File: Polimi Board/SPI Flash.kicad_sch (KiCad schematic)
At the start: 1 part, among them IC1 M95512-RMN6P

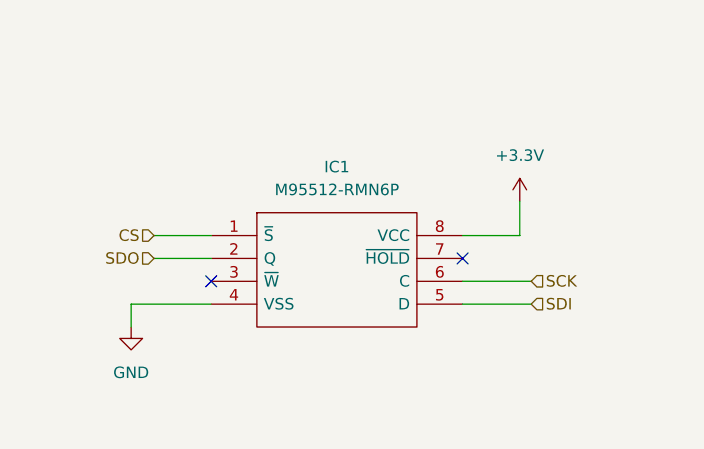
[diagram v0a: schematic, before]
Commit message: Fatte modifiche
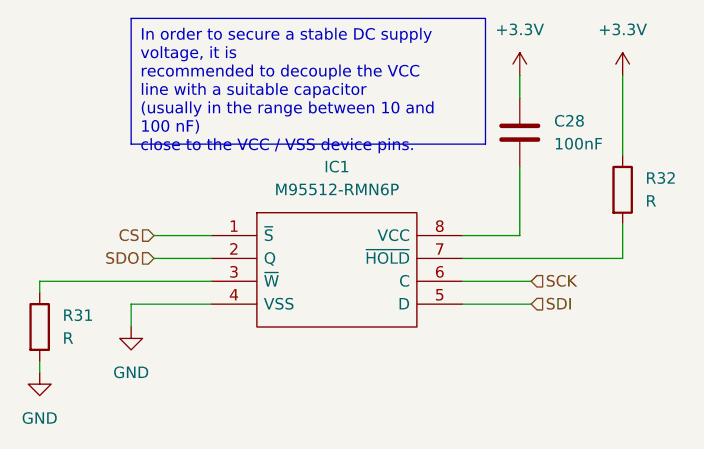
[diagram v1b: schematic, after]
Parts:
- added C28: 100nF, symbol Device:C
- added R31, R32: R, symbol Device:R
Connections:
- net +3.3V: now also C28.1, R32.1; no longer IC1.8 (VCC)
- net GND: now also R31.2
- net at IC1.3 (~{W}): now also R31.1
- net at IC1.7 (~{HOLD}): now also R32.2
- new net: C28.2, IC1.8 (VCC)
- no-connect marks 2 -> 0
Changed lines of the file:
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@@
   (title_block
     (title "Polimi Board ")
-    (date "2024-04-24")
-    (rev "1.0")
+    (date "2024-04-29")
+    (rev "2.0")
     (company "Politecnico di Milano")
     (comment 1 "Embedded Systems Project")
     (comment 2 "ing. Zaccaria Eliseo Carrettoni")
   )
-  (no_connect (at 125.73 92.71))
-  (no_connect (at 153.67 90.17))
+  (wire (pts (xy 153.67 90.17) (xy 171.45 90.17))
+    (stroke (width 0) (type default))
+  )
   (wire (pts (xy 153.67 87.63) (xy 160.02 87.63))
     (stroke (width 0) (type default))
@@
     (stroke (width 0) (type default))
   )
+  (wire (pts (xy 171.45 90.17) (xy 171.45 86.36))
+    (stroke (width 0) (type default))
+  )
+  (wire (pts (xy 106.68 101.6) (xy 106.68 102.87))
+    (stroke (width 0) (type default))
+  )
+  (wire (pts (xy 106.68 93.98) (xy 106.68 92.71))
+    (stroke (width 0) (type default))
+  )
+  (wire (pts (xy 171.45 69.85) (xy 171.45 78.74))
+    (stroke (width 0) (type default))
+  )
   (wire (pts (xy 119.38 87.63) (xy 125.73 87.63))
     (stroke (width 0) (type default))
@@
     (stroke (width 0) (type default))
   )
-  (wire (pts (xy 160.02 83.82) (xy 160.02 87.63))
+  (wire (pts (xy 160.02 72.39) (xy 160.02 69.85))
+    (stroke (width 0) (type default))
+  )
+  (wire (pts (xy 106.68 92.71) (xy 125.73 92.71))
+    (stroke (width 0) (type default))
+  )
+  (wire (pts (xy 160.02 80.01) (xy 160.02 87.63))
     (stroke (width 0) (type default))
   )
   (wire (pts (xy 116.84 97.79) (xy 116.84 95.25))
     (stroke (width 0) (type default))
+  )
+  (text_box "In order to secure a stable DC supply voltage, it is\nrecommended to decouple the VCC line with a suitable capacitor (usually in the range between 10 and 100 nF)\nclose to the VCC / VSS device pins."
+    (at 116.84 63.5 0) (size 39.37 13.97)
+    (stroke (width 0) (type default))
+    (fill (type none))
+    (effects (font (size 1.27 1.27)) (justify left top))
   )
   (hierarchical_label "SDI" (shape input) (at 161.29 95.25 0) (fields_autoplaced)
@@
         (path "/319fe76e-1f98-44b3-99b0-af1a9ad7322c/6ede4352-cbae-4369-81ad-e8e15f2edc14"
           (reference "#PWR018") (unit 1)
-        )
-      )
-    )
-  )
-  (symbol (lib_id "power:+3.3V") (at 160.02 83.82 0) (unit 1)
-    (in_bom yes) (on_board yes) (dnp no) (fields_autoplaced)
-    (property "Reference" "#PWR053" (at 160.02 87.63 0)
-      (effects (font (size 1.27 1.27)) hide)
-    )
-    (property "Value" "+3.3V" (at 160.02 78.74 0)
-      (effects (font (size 1.27 1.27)))
-    )
-    (property "Footprint" "" (at 160.02 83.82 0)
-      (effects (font (size 1.27 1.27)) hide)
-    )
-    (property "Datasheet" "" (at 160.02 83.82 0)
-      (effects (font (size 1.27 1.27)) hide)
-    )
-    (pin "1")
-    (instances
-      (project "Polimi Board"
-        (path "/319fe76e-1f98-44b3-99b0-af1a9ad7322c/6ede4352-cbae-4369-81ad-e8e15f2edc14"
-          (reference "#PWR053") (unit 1)
         )
       )
@@
         )
       )
+    )
+  )
+  (symbol (lib_id "Device:C") (at 160.02 76.2 0) (unit 1)
+    (in_bom yes) (on_board yes) (dnp no) (fields_autoplaced)
+    (property "Reference" "C28" (at 163.83 74.93 0)
+      (effects (font (size 1.27 1.27)) (justify left))
+    )
+    (property "Value" "100nF" (at 163.83 77.47 0)
+      (effects (font (size 1.27 1.27)) (justify left))
+    )
+    (property "Footprint" "" (at 160.9852 80.01 0)
+      (effects (font (size 1.27 1.27)) hide)
+    )
+    (property "Datasheet" "~" (at 160.02 76.2 0)
+      (effects (font (size 1.27 1.27)) hide)
+    )
+    (pin "2")
+    (pin "1")
+    (instances
+      (project "Polimi Board"
+        (path "/319fe76e-1f98-44b3-99b0-af1a9ad7322c/6ede4352-cbae-4369-81ad-e8e15f2edc14"
+          (reference "C28") (unit 1)
+        )
+      )
+    )
+  )
+  (symbol (lib_id "Device:R") (at 106.68 97.79 0) (unit 1)
+    (in_bom yes) (on_board yes) (dnp no) (fields_autoplaced)
+    (property "Reference" "R31" (at 109.22 96.52 0)
+      (effects (font (size 1.27 1.27)) (justify left))
+    )
+    (property "Value" "R" (at 109.22 99.06 0)
+      (effects (font (size 1.27 1.27)) (justify left))
+    )
+    (property "Footprint" "" (at 104.902 97.79 90)
+      (effects (font (size 1.27 1.27)) hide)
+    )
+    (property "Datasheet" "~" (at 106.68 97.79 0)
+      (effects (font (size 1.27 1.27)) hide)
+    )
+    (pin "1")
+    (pin "2")
+    (instances
+      (project "Polimi Board"
+        (path "/319fe76e-1f98-44b3-99b0-af1a9ad7322c/6ede4352-cbae-4369-81ad-e8e15f2edc14"
+          (reference "R31") (unit 1)
+        )
+      )
+    )
+  )
+  (symbol (lib_id "power:+3.3V") (at 160.02 69.85 0) (unit 1)
+    (in_bom yes) (on_board yes) (dnp no) (fields_autoplaced)
+    (property "Reference" "#PWR025" (at 160.02 73.66 0)
+      (effects (font (size 1.27 1.27)) hide)
+    )
+    (property "Value" "+3.3V" (at 160.02 64.77 0)
+      (effects (font (size 1.27 1.27)))
+    )
+    (property "Footprint" "" (at 160.02 69.85 0)
+      (effects (font (size 1.27 1.27)) hide)
+    )
+    (property "Datasheet" "" (at 160.02 69.85 0)
+      (effects (font (size 1.27 1.27)) hide)
+    )
+    (pin "1")
+    (instances
+      (project "Polimi Board"
+        (path "/319fe76e-1f98-44b3-99b0-af1a9ad7322c/6ede4352-cbae-4369-81ad-e8e15f2edc14"
+          (reference "#PWR025") (unit 1)
+        )
+      )
+    )
+  )
+  (symbol (lib_id "power:GND") (at 106.68 102.87 0) (unit 1)
+    (in_bom yes) (on_board yes) (dnp no) (fields_autoplaced)
+    (property "Reference" "#PWR069" (at 106.68 109.22 0)
+      (effects (font (size 1.27 1.27)) hide)
+    )
+    (property "Value" "GND" (at 106.68 107.95 0)
+      (effects (font (size 1.27 1.27)))
+    )
+    (property "Footprint" "" (at 106.68 102.87 0)
+      (effects (font (size 1.27 1.27)) hide)
+    )
+    (property "Datasheet" "" (at 106.68 102.87 0)
+      (effects (font (size 1.27 1.27)) hide)
+    )
+    (pin "1")
+    (instances
+      (project "Polimi Board"
+        (path "/319fe76e-1f98-44b3-99b0-af1a9ad7322c/6ede4352-cbae-4369-81ad-e8e15f2edc14"
+          (reference "#PWR069") (unit 1)
+        )
+      )
+    )
+  )
+  (symbol (lib_id "Device:R") (at 171.45 82.55 0) (unit 1)
+    (in_bom yes) (on_board yes) (dnp no) (fields_autoplaced)
+    (property "Reference" "R32" (at 173.99 81.28 0)
+      (effects (font (size 1.27 1.27)) (justify left))
+    )
+    (property "Value" "R" (at 173.99 83.82 0)
+      (effects (font (size 1.27 1.27)) (justify left))
+    )
+    (property "Footprint" "" (at 169.672 82.55 90)
+      (effects (font (size 1.27 1.27)) hide)
+    )
+    (property "Datasheet" "~" (at 171.45 82.55 0)
+      (effects (font (size 1.27 1.27)) hide)
+    )
+    (pin "1")
+    (pin "2")
+    (instances
+      (project "Polimi Board"
+        (path "/319fe76e-1f98-44b3-99b0-af1a9ad7322c/6ede4352-cbae-4369-81ad-e8e15f2edc14"
+          (reference "R32") (unit 1)
+        )
+      )
+    )
+  )
+  (symbol (lib_id "power:+3.3V") (at 171.45 69.85 0) (unit 1)
+    (in_bom yes) (on_board yes) (dnp no) (fields_autoplaced)
+    (property "Reference" "#PWR090" (at 171.45 73.66 0)
+      (effects (font (size 1.27 1.27)) hide)
+    )
+    (property "Value" "+3.3V" (at 171.45 64.77 0)
+      (effects (font (size 1.27 1.27)))
+    )
+    (property "Footprint" "" (at 171.45 69.85 0)
+      (effects (font (size 1.27 1.27)) hide)
+    )
+    (property "Datasheet" "" (at 171.45 69.85 0)
+      (effects (font (size 1.27 1.27)) hide)
+    )
+    (pin "1")
+    (instances
+      (project "Polimi Board"
+        (path "/319fe76e-1f98-44b3-99b0-af1a9ad7322c/6ede4352-cbae-4369-81ad-e8e15f2edc14"
+          (reference "#PWR090") (unit 1)
+        )
+      )
